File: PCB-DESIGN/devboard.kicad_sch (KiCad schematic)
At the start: 34 parts, among them J1 USB_C_Receptacle_USB2.0_14P, J2 Conn_01x20, J3 Conn_01x20, J4 Conn_01x03, SW1 SW_Push, U1 RP2040, U2 MCP1700x-330xxTT, U3 W25Q16JVUXIQ TR, Y1 12 MHz

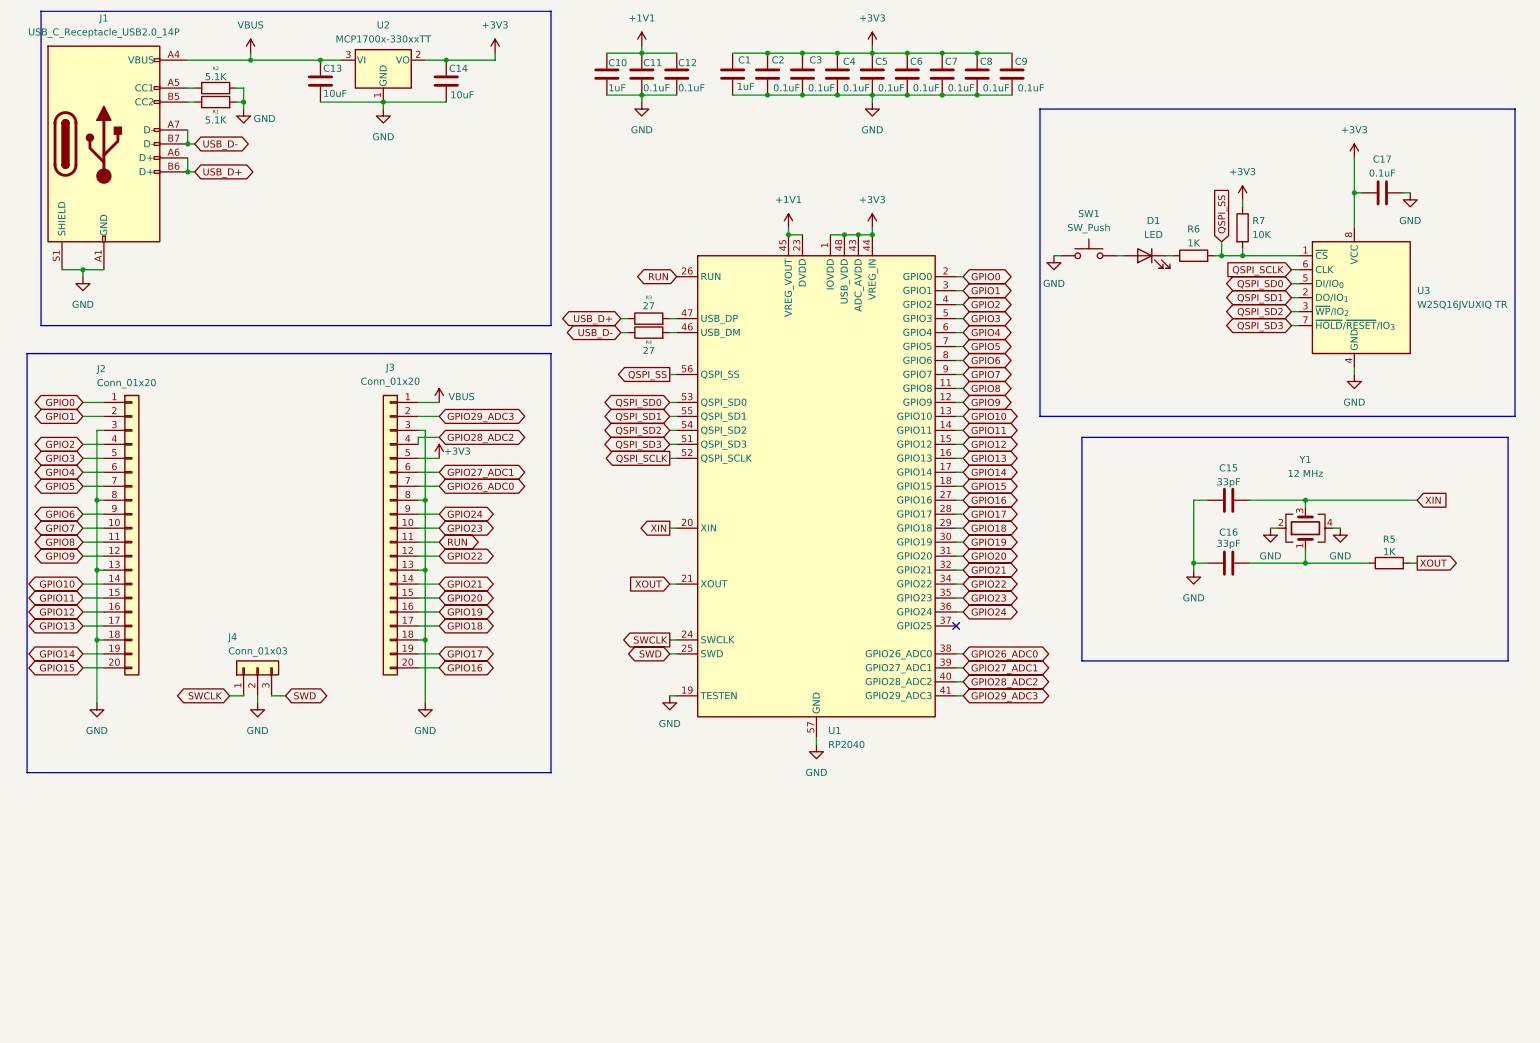
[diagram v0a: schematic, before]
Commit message: Add files via upload
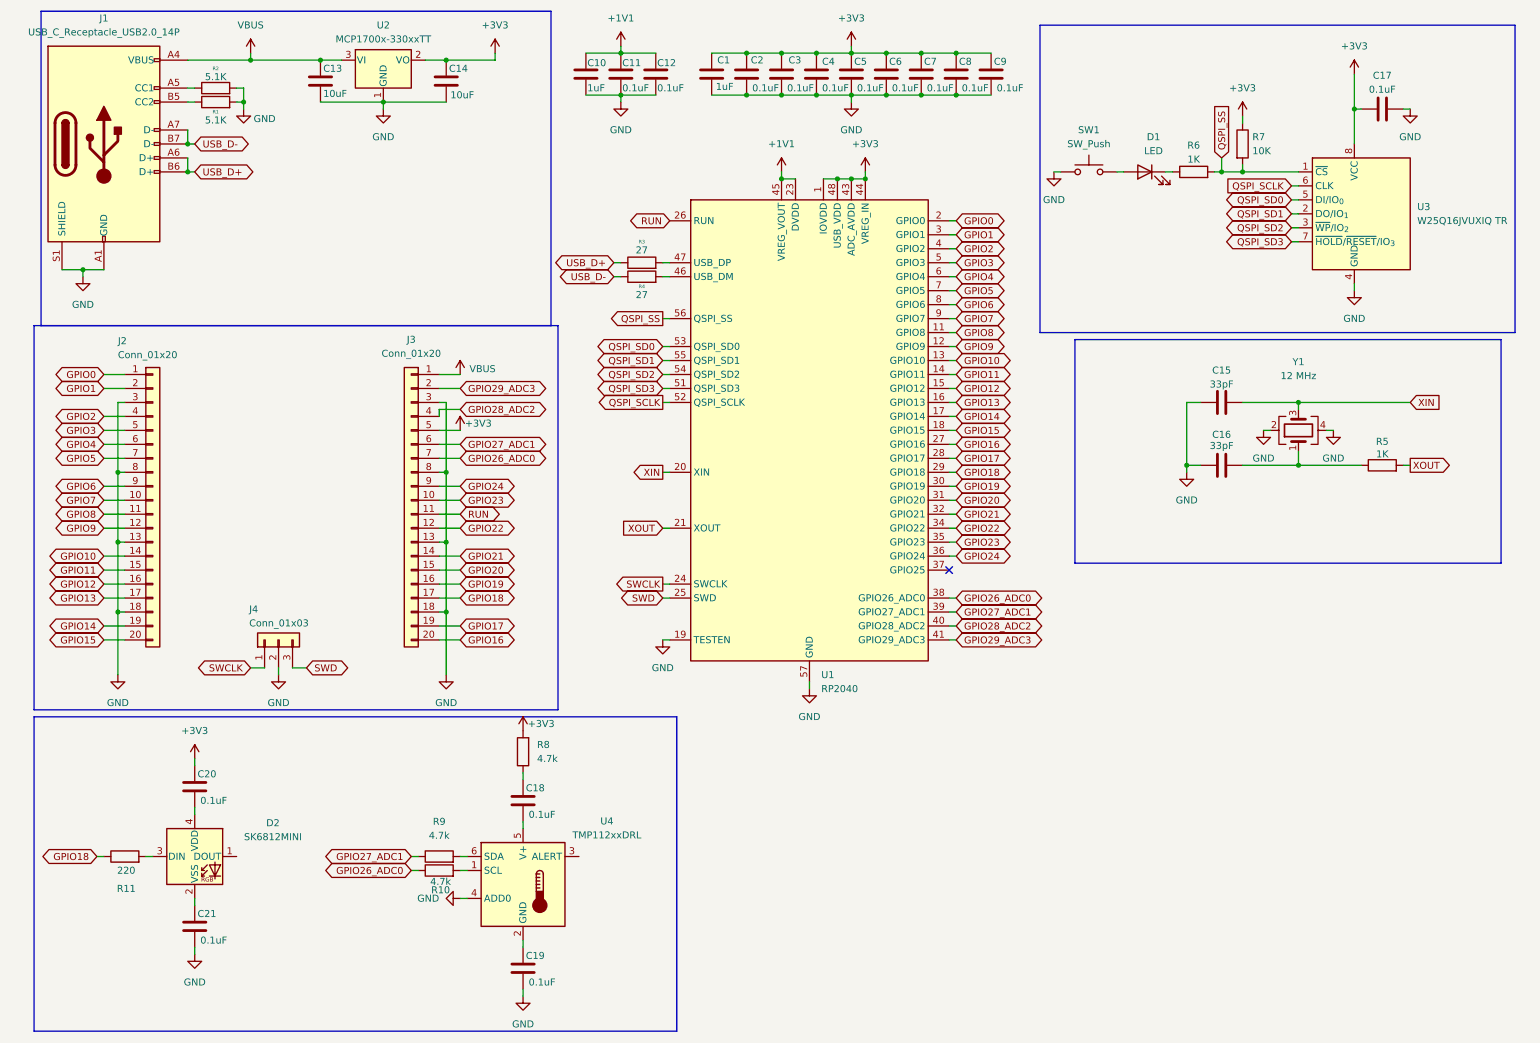
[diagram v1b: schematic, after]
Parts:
- added C18, C19, C20, C21: 0.1uF, Capacitor_SMD:C_0402_1005Metric, symbol Device:C
- added D2: SK6812MINI, LED_SMD:LED_SK6812MINI_PLCC4_3.5x3.5mm_P1.75mm, symbol LED:SK6812MINI
- added R10, R8, R9: 4.7k, Resistor_SMD:R_0402_1005Metric, symbol Device:R
- added R11: 220, Resistor_SMD:R_0402_1005Metric, symbol Device:R
- added U4: TMP112xxDRL, Package_TO_SOT_SMD:SOT-563, symbol Sensor_Temperature:TMP112xxDRL
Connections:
- net +3V3: now also C20.1, R8.2
- net GND: now also C19.2, C21.2, U4.4 (ADD0)
- net GPIO18: now also R11.1
- net GPIO26_ADC0: now also R10.1
- net GPIO27_ADC1: now also R9.1
- new net: C18.1, R8.1
- new net: R9.2, U4.6 (SDA)
- new net: C21.1, D2.2 (VSS)
- new net: D2.3 (DIN), R11.2
- new net: C20.2, D2.4 (VDD)
- new net: R10.2, U4.1 (SCL)
- new net: C19.1, U4.2 (GND)
- new net: C18.2, U4.5 (V+)
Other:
- moved on the sheet: C1, C10, C11, C12, C15, C16, C17, C2, C3, C4, C5, C6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
